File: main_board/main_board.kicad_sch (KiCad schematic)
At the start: 6 parts, among them J13 Conn_01x16, U1 Pico, U2 MPR121QR2

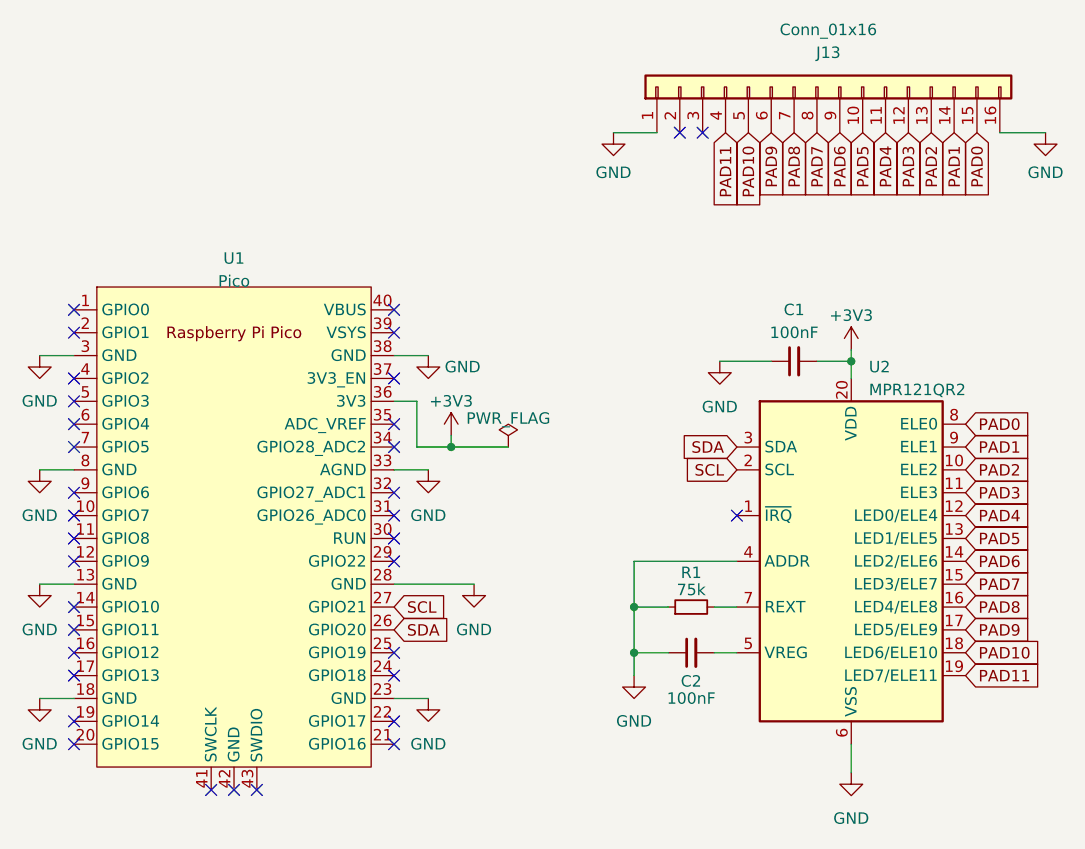
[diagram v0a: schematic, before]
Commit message: Add code.py, update gerbers/prod files
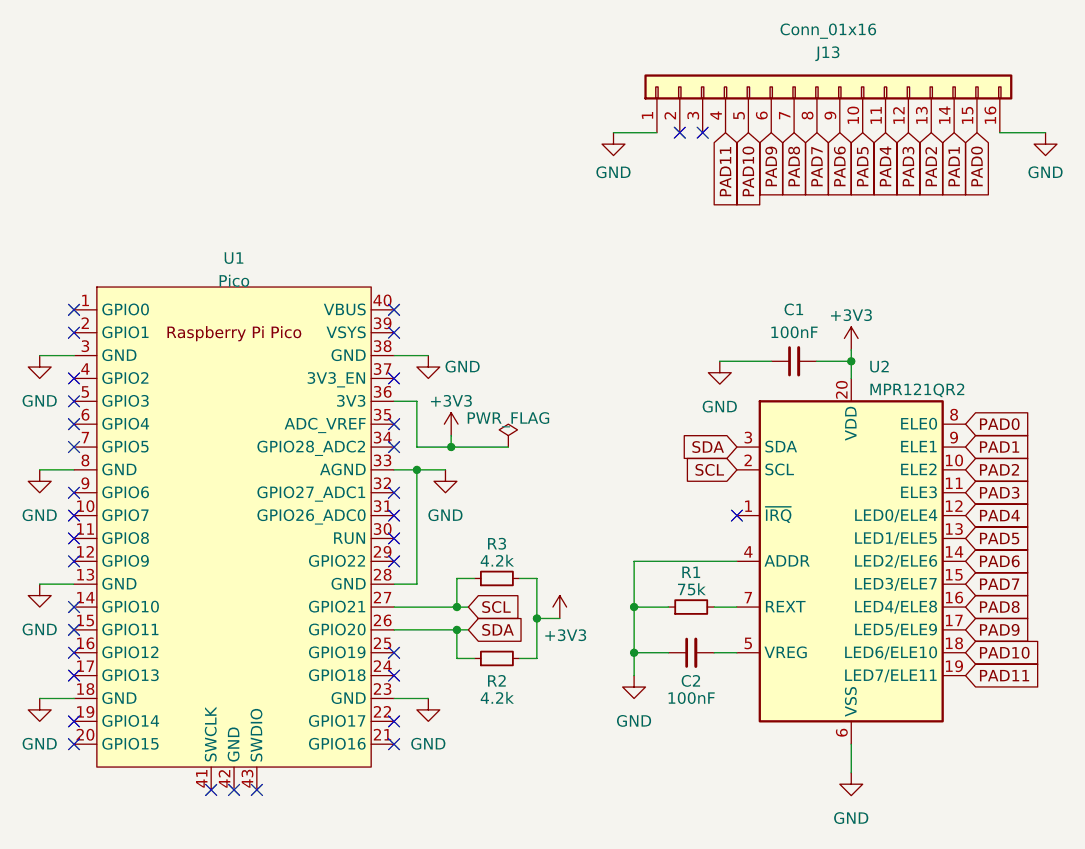
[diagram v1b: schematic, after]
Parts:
- added R2, R3: 4.2k, Resistor_SMD:R_0805_2012Metric_Pad1.20x1.40mm_HandSolder, symbol Device:R_Small
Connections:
- net +3V3: now also R2.2, R3.2
- net SCL: now also R3.1
- net SDA: now also R2.1
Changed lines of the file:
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@@
   (junction (at 163.195 109.22) (diameter 0) (color 0 0 0 0)
   )
+  (junction (at 139.065 88.9) (diameter 0) (color 0 0 0 0)
+  )
   (junction (at 187.325 76.835) (diameter 0) (color 0 0 0 0)
   )
+  (junction (at 143.51 104.14) (diameter 0) (color 0 0 0 0)
+  )
   (junction (at 163.195 104.14) (diameter 0) (color 0 0 0 0)
   )
   (junction (at 142.875 86.36) (diameter 0) (color 0 0 0 0)
+  )
+  (junction (at 152.4 105.41) (diameter 0) (color 0 0 0 0)
+  )
+  (junction (at 143.51 106.68) (diameter 0) (color 0 0 0 0)
   )
   (no_connect (at 100.965 78.74))
@@
     (stroke (width 0) (type default))
   )
+  (wire (pts (xy 152.4 105.41) (xy 154.94 105.41))
+    (stroke (width 0) (type default))
+  )
+  (wire (pts (xy 152.4 100.965) (xy 152.4 105.41))
+    (stroke (width 0) (type default))
+  )
   (wire (pts (xy 142.875 86.36) (xy 149.225 86.36))
     (stroke (width 0) (type default))
   )
-  (wire (pts (xy 136.525 101.6) (xy 145.415 101.6))
+  (wire (pts (xy 144.78 106.68) (xy 143.51 106.68))
+    (stroke (width 0) (type default))
+  )
+  (wire (pts (xy 139.065 101.6) (xy 139.065 88.9))
     (stroke (width 0) (type default))
   )
@@
     (stroke (width 0) (type default))
   )
+  (wire (pts (xy 136.525 101.6) (xy 139.065 101.6))
+    (stroke (width 0) (type default))
+  )
   (wire (pts (xy 174.625 99.06) (xy 163.195 99.06))
     (stroke (width 0) (type default))
@@
     (stroke (width 0) (type default))
   )
+  (wire (pts (xy 143.51 109.855) (xy 145.415 109.855))
+    (stroke (width 0) (type default))
+  )
+  (wire (pts (xy 152.4 105.41) (xy 152.4 109.855))
+    (stroke (width 0) (type default))
+  )
+  (wire (pts (xy 143.51 106.68) (xy 136.525 106.68))
+    (stroke (width 0) (type default))
+  )
   (wire (pts (xy 97.155 76.2) (xy 100.965 76.2))
     (stroke (width 0) (type default))
   )
+  (wire (pts (xy 143.51 100.965) (xy 143.51 104.14))
+    (stroke (width 0) (type default))
+  )
   (wire (pts (xy 97.155 101.6) (xy 100.965 101.6))
     (stroke (width 0) (type default))
@@
     (stroke (width 0) (type default))
   )
+  (wire (pts (xy 152.4 109.855) (xy 150.495 109.855))
+    (stroke (width 0) (type default))
+  )
   (wire (pts (xy 142.875 85.09) (xy 142.875 86.36))
     (stroke (width 0) (type default))
   )
-  (wire (pts (xy 136.525 88.9) (xy 140.335 88.9))
+  (wire (pts (xy 139.065 88.9) (xy 142.24 88.9))
+    (stroke (width 0) (type default))
+  )
+  (wire (pts (xy 136.525 88.9) (xy 139.065 88.9))
+    (stroke (width 0) (type default))
+  )
+  (wire (pts (xy 143.51 104.14) (xy 136.525 104.14))
+    (stroke (width 0) (type default))
+  )
+  (wire (pts (xy 145.415 100.965) (xy 143.51 100.965))
     (stroke (width 0) (type default))
   )
@@
     (stroke (width 0) (type default))
   )
+  (wire (pts (xy 150.495 100.965) (xy 152.4 100.965))
+    (stroke (width 0) (type default))
+  )
+  (wire (pts (xy 144.78 104.14) (xy 143.51 104.14))
+    (stroke (width 0) (type default))
+  )
   (wire (pts (xy 165.735 51.435) (xy 160.909 51.435))
     (stroke (width 0) (type default))
@@
     (stroke (width 0) (type default))
   )
+  (wire (pts (xy 143.51 106.68) (xy 143.51 109.855))
+    (stroke (width 0) (type default))
+  )
   (global_label "PAD3" (shape input) (at 193.675 51.435 270) (fields_autoplaced)
     (effects (font (size 1.27 1.27)) (justify right))
@@
     )
   )
-  (global_label "SCL" (shape input) (at 136.525 104.14 0) (fields_autoplaced)
-    (effects (font (size 1.27 1.27)) (justify left))
-    (property "Intersheetrefs" "${INTERSHEET_REFS}" (at 142.9384 104.14 0)
+  (global_label "SCL" (shape input) (at 144.78 104.14 0) (fields_autoplaced)
+    (effects (font (size 1.27 1.27)) (justify left))
+    (property "Intersheetrefs" "${INTERSHEET_REFS}" (at 151.1934 104.14 0)
       (effects (font (size 1.27 1.27)) (justify left) hide)
     )
@@
     )
   )
-  (global_label "SDA" (shape input) (at 136.525 106.68 0) (fields_autoplaced)
-    (effects (font (size 1.27 1.27)) (justify left))
-    (property "Intersheetrefs" "${INTERSHEET_REFS}" (at 142.9989 106.68 0)
+  (global_label "SDA" (shape input) (at 144.78 106.68 0) (fields_autoplaced)
+    (effects (font (size 1.27 1.27)) (justify left))
+    (property "Intersheetrefs" "${INTERSHEET_REFS}" (at 151.2539 106.68 0)
       (effects (font (size 1.27 1.27)) (justify left) hide)
     )
@@
     )
   )
-  (symbol (lib_id "power:GND") (at 145.415 101.6 0) (unit 1)
-    (in_bom yes) (on_board yes) (dnp no) (fields_autoplaced)
-    (property "Reference" "#PWR07" (at 145.415 107.95 0)
-      (effects (font (size 1.27 1.27)) hide)
-    )
-    (property "Value" "GND" (at 145.415 106.68 0)
-      (effects (font (size 1.27 1.27)))
-    )
-    (property "Footprint" "" (at 145.415 101.6 0)
-      (effects (font (size 1.27 1.27)) hide)
-    )
-    (property "Datasheet" "" (at 145.415 101.6 0)
+  (symbol (lib_id "Device:C_Small") (at 180.975 76.835 90) (unit 1)
+    (in_bom yes) (on_board yes) (dnp no) (fields_autoplaced)
+    (property "Reference" "C1" (at 180.9813 71.12 90)
+      (effects (font (size 1.27 1.27)))
+    )
+    (property "Value" "100nF" (at 180.9813 73.66 90)
+      (effects (font (size 1.27 1.27)))
+    )
+    (property "Footprint" "Capacitor_SMD:C_0805_2012Metric_Pad1.18x1.45mm_HandSolder" (at 180.975 76.835 0)
+      (effects (font (size 1.27 1.27)) hide)
+    )
+    (property "Datasheet" "~" (at 180.975 76.835 0)
+      (effects (font (size 1.27 1.27)) hide)
+    )
+    (property "LCSC" "C49678" (at 180.975 76.835 0)
+      (effects (font (size 1.27 1.27)) hide)
+    )
+    (pin "1")
+    (pin "2")
+    (instances
+      (project "main_board"
+        (path "/4a11fb4e-37e4-46fa-b38a-c052d00a21bc"
+          (reference "C1") (unit 1)
+        )
+      )
+    )
+  )
+  (symbol (lib_id "power:+3V3") (at 154.94 105.41 0) (unit 1)
+    (in_bom yes) (on_board yes) (dnp no)
+    (property "Reference" "#PWR07" (at 154.94 109.22 0)
+      (effects (font (size 1.27 1.27)) hide)
+    )
+    (property "Value" "+3V3" (at 155.575 107.315 0)
+      (effects (font (size 1.27 1.27)))
+    )
+    (property "Footprint" "" (at 154.94 105.41 0)
+      (effects (font (size 1.27 1.27)) hide)
+    )
+    (property "Datasheet" "" (at 154.94 105.41 0)
       (effects (font (size 1.27 1.27)) hide)
     )
@@
     )
   )
-  (symbol (lib_id "Device:C_Small") (at 180.975 76.835 90) (unit 1)
-    (in_bom yes) (on_board yes) (dnp no) (fields_autoplaced)
-    (property "Reference" "C1" (at 180.9813 71.12 90)
-      (effects (font (size 1.27 1.27)))
-    )
-    (property "Value" "100nF" (at 180.9813 73.66 90)
-      (effects (font (size 1.27 1.27)))
-    )
-    (property "Footprint" "Capacitor_SMD:C_0805_2012Metric_Pad1.18x1.45mm_HandSolder" (at 180.975 76.835 0)
-      (effects (font (size 1.27 1.27)) hide)
-    )
-    (property "Datasheet" "~" (at 180.975 76.835 0)
-      (effects (font (size 1.27 1.27)) hide)
-    )
-    (property "LCSC" "C49678" (at 180.975 76.835 0)
-      (effects (font (size 1.27 1.27)) hide)
-    )
-    (pin "1")
-    (pin "2")
-    (instances
-      (project "main_board"
-        (path "/4a11fb4e-37e4-46fa-b38a-c052d00a21bc"
-          (reference "C1") (unit 1)
-        )
-      )
-    )
-  )
-  (symbol (lib_id "power:GND") (at 140.335 88.9 0) (unit 1)
-    (in_bom yes) (on_board yes) (dnp no) (fields_autoplaced)
-    (property "Reference" "#PWR08" (at 140.335 95.25 0)
-      (effects (font (size 1.27 1.27)) hide)
-    )
-    (property "Value" "GND" (at 140.335 93.98 0)
-      (effects (font (size 1.27 1.27)))
-    )
-    (property "Footprint" "" (at 140.335 88.9 0)
-      (effects (font (size 1.27 1.27)) hide)
-    )
-    (property "Datasheet" "" (at 140.335 88.9 0)
+  (symbol (lib_id "power:GND") (at 142.24 88.9 0) (unit 1)
+    (in_bom yes) (on_board yes) (dnp no) (fields_autoplaced)
+    (property "Reference" "#PWR08" (at 142.24 95.25 0)
+      (effects (font (size 1.27 1.27)) hide)
+    )
+    (property "Value" "GND" (at 142.24 93.98 0)
+      (effects (font (size 1.27 1.27)))
+    )
+    (property "Footprint" "" (at 142.24 88.9 0)
+      (effects (font (size 1.27 1.27)) hide)
+    )
+    (property "Datasheet" "" (at 142.24 88.9 0)
       (effects (font (size 1.27 1.27)) hide)
     )
@@
     )
   )
+  (symbol (lib_id "Device:R_Small") (at 147.955 109.855 90) (unit 1)
+    (in_bom yes) (on_board yes) (dnp no)
+    (property "Reference" "R2" (at 147.955 112.395 90)
+      (effects (font (size 1.27 1.27)))
+    )
+    (property "Value" "4.2k" (at 147.955 114.3 90)
+      (effects (font (size 1.27 1.27)))
+    )
+    (property "Footprint" "Resistor_SMD:R_0805_2012Metric_Pad1.20x1.40mm_HandSolder" (at 147.955 109.855 0)
+      (effects (font (size 1.27 1.27)) hide)
+    )
+    (property "Datasheet" "~" (at 147.955 109.855 0)
+      (effects (font (size 1.27 1.27)) hide)
+    )
+    (pin "1")
+    (pin "2")
+    (instances
+      (project "main_board"
+        (path "/4a11fb4e-37e4-46fa-b38a-c052d00a21bc"
+          (reference "R2") (unit 1)
+        )
+      )
+    )
+  )
   (symbol (lib_id "power:GND") (at 97.155 114.3 0) (unit 1)
     (in_bom yes) (on_board yes) (dnp no) (fields_autoplaced)
@@
         )
       )
+    )
+  )
+  (symbol (lib_id "Device:R_Small") (at 147.955 100.965 90) (unit 1)
+    (in_bom yes) (on_board yes) (dnp no)
+    (property "Reference" "R3" (at 147.955 97.155 90)
+      (effects (font (size 1.27 1.27)))
+    )
+    (property "Value" "4.2k" (at 147.955 99.06 90)
+      (effects (font (size 1.27 1.27)))
+    )
+    (property "Footprint" "Resistor_SMD:R_0805_2012Metric_Pad1.20x1.40mm_HandSolder" (at 147.955 100.965 0)
+      (effects (font (size 1.27 1.27)) hide)
+    )
+    (property "Datasheet" "~" (at 147.955 100.965 0)
+      (effects (font (size 1.27 1.27)) hide)
+    )
+    (pin "1")
+    (pin "2")
+    (instances
+      (project "main_board"
+        (path "/4a11fb4e-37e4-46fa-b38a-c052d00a21bc"
+          (reference "R3") (unit 1)
+        )
+      )
